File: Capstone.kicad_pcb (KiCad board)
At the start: 2 copper layers, 21 parts, among them U1 XIAO-ESP32-S3-DIP, U2 LM358, U3 LM358, U4 LM358, U5 LM358

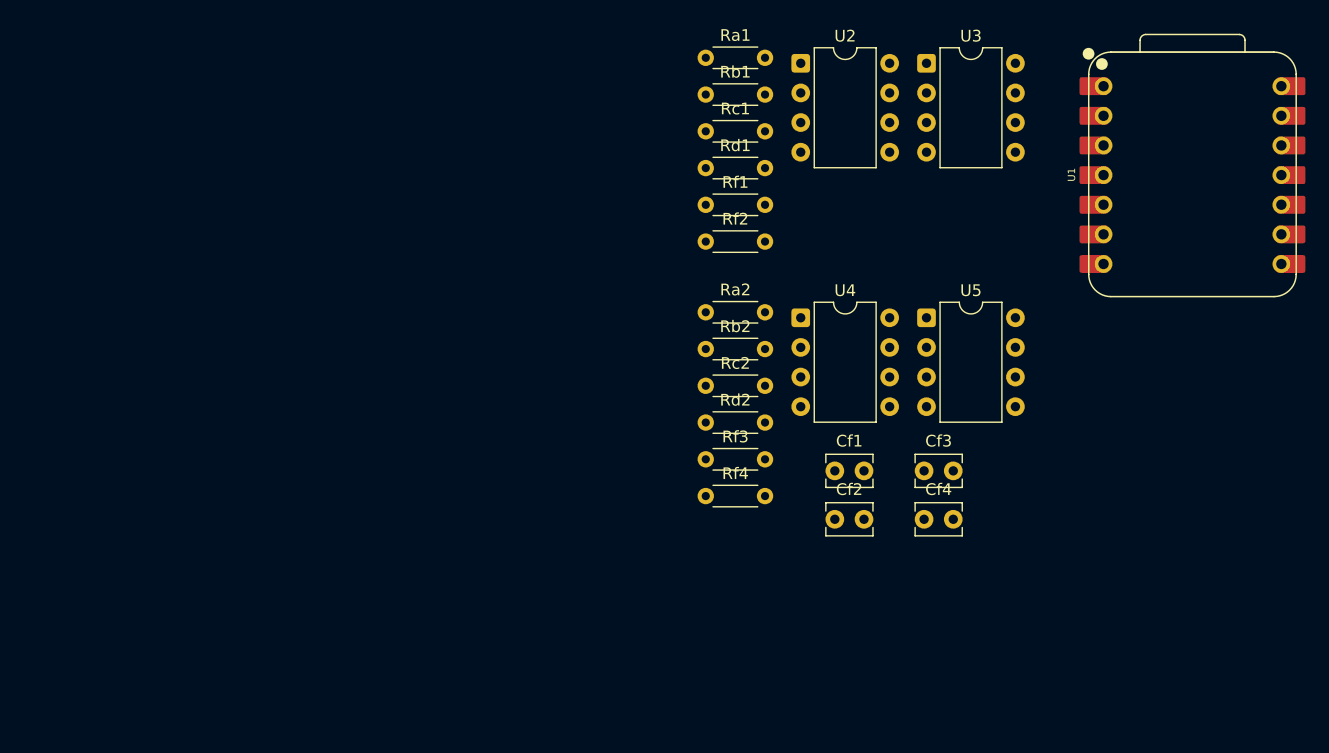
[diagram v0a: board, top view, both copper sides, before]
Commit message: PCB designed rev1.0
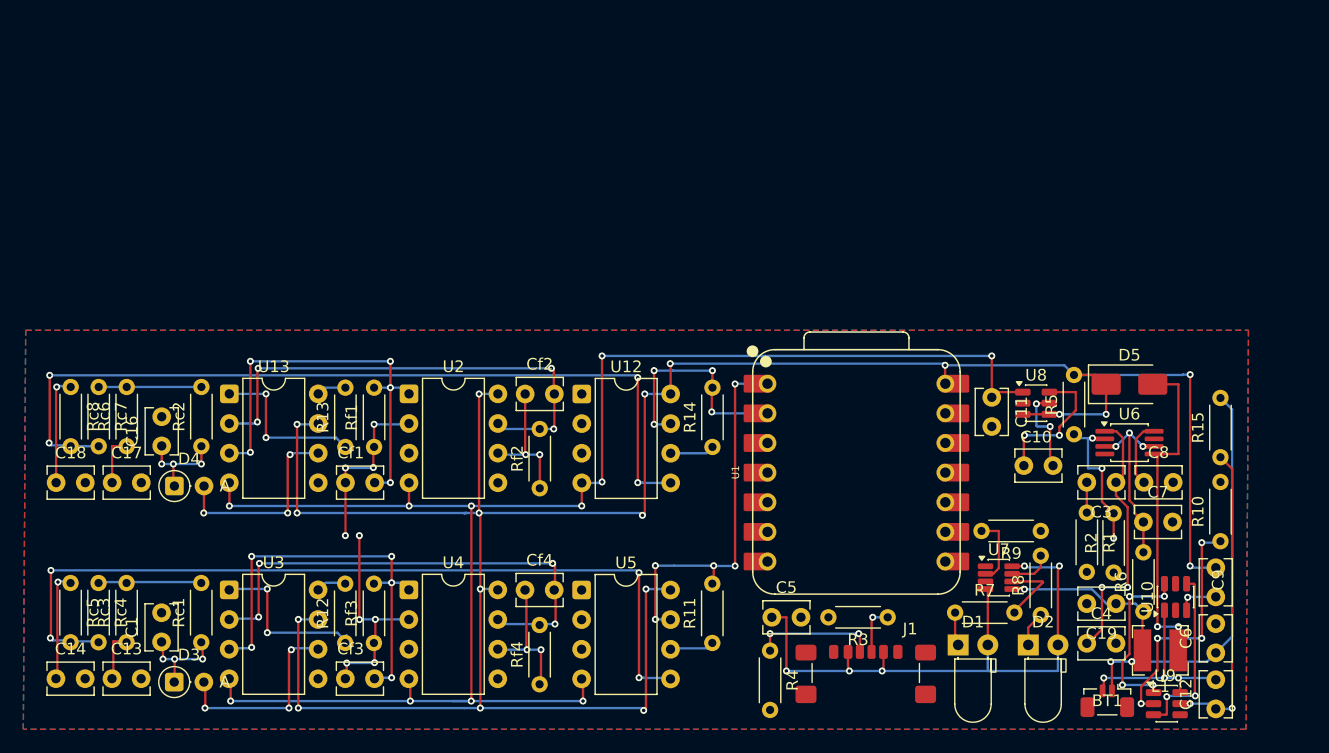
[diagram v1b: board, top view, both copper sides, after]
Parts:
- removed Ra1, Ra2, Rb1, Rb2, Rd1, Rd2: 100k, Resistor_THT:R_Axial_DIN0204_L3.6mm_D1.6mm_P5.08mm_Horizontal
- added BT1: Battery, Connector_JST:JST_SUR_BM02B-SURS-TF_1x02-1MP_P0.80mm_Vertical, F.Cu at (176.7, 125.5)
- added C1: 100p, Capacitor_THT:C_Disc_D3.8mm_W2.6mm_P2.50mm, F.Cu at (95.6, 120.5)
- added C10: 1uF, Capacitor_THT:C_Disc_D3.8mm_W2.6mm_P2.50mm, F.Cu at (172.1, 105.4)
- added C11: 2.2uF, Capacitor_THT:C_Disc_D3.8mm_W2.6mm_P2.50mm, F.Cu at (166.8, 99.5)
- added C12: 100nF, Capacitor_THT:C_Disc_D3.8mm_W2.6mm_P2.50mm, F.Cu at (186.0, 126.2)
- added C13: 100p, Capacitor_THT:C_Disc_D3.8mm_W2.6mm_P2.50mm, F.Cu at (91.4, 123.7)
- added C14: 100p, Capacitor_THT:C_Disc_D3.8mm_W2.6mm_P2.50mm, F.Cu at (86.6, 123.7)
- added C16: 100p, Capacitor_THT:C_Disc_D3.8mm_W2.6mm_P2.50mm, F.Cu at (95.7, 103.7)
- added C17: 100p, Capacitor_THT:C_Disc_D3.8mm_W2.6mm_P2.50mm, F.Cu at (91.4, 106.9)
- added C18: 100p, Capacitor_THT:C_Disc_D3.8mm_W2.6mm_P2.50mm, F.Cu at (86.6, 106.9)
- added C19: 10uF, Capacitor_THT:C_Disc_D3.8mm_W2.6mm_P2.50mm, F.Cu at (177.4, 117.2)
- added C3: 3900pF, Capacitor_THT:C_Disc_D3.8mm_W2.6mm_P2.50mm, F.Cu at (177.4, 106.8)
- added C4: 10pF, Capacitor_THT:C_Disc_D3.8mm_W2.6mm_P2.50mm, F.Cu at (174.9, 120.6)
- added C5: 4.7uF, Capacitor_THT:C_Disc_D3.8mm_W2.6mm_P2.50mm, F.Cu at (147.9, 118.4)
- added C6: 10uF, Capacitor_THT:C_Disc_D3.8mm_W2.6mm_P2.50mm, F.Cu at (186.0, 121.5)
- added C7: 1uF, Capacitor_THT:C_Disc_D3.8mm_W2.6mm_P2.50mm, F.Cu at (179.8, 110.2)
- added C8: 10nF, Capacitor_THT:C_Disc_D3.8mm_W2.6mm_P2.50mm, F.Cu at (179.8, 106.8)
- added C9: 10uF, Capacitor_THT:C_Disc_D3.8mm_W2.6mm_P2.50mm, F.Cu at (186.0, 114.2)
- added D1: LED, LED_THT:LED_D3.0mm_Horizontal_O1.27mm_Z6.0mm, F.Cu at (163.9, 120.8)
- added D2: LED, LED_THT:LED_D3.0mm_Horizontal_O1.27mm_Z6.0mm, F.Cu at (169.9, 120.8)
- added D3: 1N34A, Diode_THT:D_DO-35_SOD27_P2.54mm_Vertical_AnodeUp, F.Cu at (96.7, 124.0)
- added D4: 1N34A, Diode_THT:D_DO-35_SOD27_P2.54mm_Vertical_AnodeUp, F.Cu at (96.7, 107.2)
- added D5: B240A, Diode_SMD:D_SMA, F.Cu at (178.6, 98.4)
- added J1: USB_C_Receptacle_PowerOnly_6P, Connector_USB:USB_C_Receptacle_GCT_USB4135-GF-A_6P_TopMnt_Horizontal, F.Cu at (156.0, 124.4)
- added L1: 3.9uH, Inductor_SMD:L_Bourns-SRN4018, F.Cu at (181.2, 121.2)
- added R1: 4.75k, Resistor_THT:R_Axial_DIN0204_L3.6mm_D1.6mm_P5.08mm_Horizontal, F.Cu at (174.9, 109.4)
- added R10: 1k, Resistor_THT:R_Axial_DIN0204_L3.6mm_D1.6mm_P5.08mm_Horizontal, F.Cu at (186.4, 111.9)
- added R11: 1k, Resistor_THT:R_Axial_DIN0204_L3.6mm_D1.6mm_P5.08mm_Horizontal, F.Cu at (142.8, 120.6)
- added R12: 500, Resistor_THT:R_Axial_DIN0204_L3.6mm_D1.6mm_P5.08mm_Horizontal, F.Cu at (111.4, 120.6)
- added R13: 500, Resistor_THT:R_Axial_DIN0204_L3.6mm_D1.6mm_P5.08mm_Horizontal, F.Cu at (111.4, 103.8)
- added R14: 1k, Resistor_THT:R_Axial_DIN0204_L3.6mm_D1.6mm_P5.08mm_Horizontal, F.Cu at (142.9, 103.8)
- added R15: 100R, Resistor_THT:R_Axial_DIN0204_L3.6mm_D1.6mm_P5.08mm_Horizontal, F.Cu at (186.4, 104.7)
- added R2: 33.2K, Resistor_THT:R_Axial_DIN0204_L3.6mm_D1.6mm_P5.08mm_Horizontal, F.Cu at (177.2, 114.6)
- added R3: 5.11k, Resistor_THT:R_Axial_DIN0204_L3.6mm_D1.6mm_P5.08mm_Horizontal, F.Cu at (157.9, 118.4)
- added R4: 5.11k, Resistor_THT:R_Axial_DIN0204_L3.6mm_D1.6mm_P5.08mm_Horizontal, F.Cu at (147.8, 121.3)
- added R5: 102k, Resistor_THT:R_Axial_DIN0204_L3.6mm_D1.6mm_P5.08mm_Horizontal, F.Cu at (173.8, 102.7)
- added R6: 1, Resistor_THT:R_Axial_DIN0204_L3.6mm_D1.6mm_P5.08mm_Horizontal, F.Cu at (179.8, 117.9)
- added R7: 5.11k, Resistor_THT:R_Axial_DIN0204_L3.6mm_D1.6mm_P5.08mm_Horizontal, F.Cu at (163.7, 118.0)
- added R8: 5.11k, Resistor_THT:R_Axial_DIN0204_L3.6mm_D1.6mm_P5.08mm_Horizontal, F.Cu at (171.0, 118.2)
- added R9: 5.11k, Resistor_THT:R_Axial_DIN0204_L3.6mm_D1.6mm_P5.08mm_Horizontal, F.Cu at (171.0, 111.0)
- added Rc3: 1k, Resistor_THT:R_Axial_DIN0204_L3.6mm_D1.6mm_P5.08mm_Horizontal, F.Cu at (92.6, 120.5)
- added Rc4: 100k, Resistor_THT:R_Axial_DIN0204_L3.6mm_D1.6mm_P5.08mm_Horizontal, F.Cu at (90.2, 115.5)
- added Rc5: 1k, Resistor_THT:R_Axial_DIN0204_L3.6mm_D1.6mm_P5.08mm_Horizontal, F.Cu at (87.8, 115.5)
- added Rc6: 1k, Resistor_THT:R_Axial_DIN0204_L3.6mm_D1.6mm_P5.08mm_Horizontal, F.Cu at (92.7, 103.7)
- added Rc7: 100k, Resistor_THT:R_Axial_DIN0204_L3.6mm_D1.6mm_P5.08mm_Horizontal, F.Cu at (90.3, 98.7)
- added Rc8: 1k, Resistor_THT:R_Axial_DIN0204_L3.6mm_D1.6mm_P5.08mm_Horizontal, F.Cu at (87.9, 98.7)
- added U10: ~, Package_TO_SOT_SMD:SOT-23-6, F.Cu at (182.6, 116.7)
- added U12: LM358, Package_DIP:DIP-8_W7.62mm, F.Cu at (131.7, 99.3)
- added U13: INA128, Package_DIP:DIP-8_W7.62mm, F.Cu at (101.5, 99.2)
- added U6: ADP1613ARMZ-R7, Package_SO:MSOP-8_3x3mm_P0.65mm, F.Cu at (178.6, 103.4)
- added U7: ~, Package_TO_SOT_SMD:SOT-23-8, F.Cu at (167.4, 115.0)
- added U8: LM2776, Package_TO_SOT_SMD:SOT-23-6, F.Cu at (170.6, 100.0)
- added U9: ~, Package_TO_SOT_SMD:SOT-23-6, F.Cu at (181.8, 125.8)
- Cf1, Cf3: value 10p -> 2p
- U3: value LM358 -> INA128
- moved U3 74.9 mm to (101.4, 116.0)
- moved Rc1 61.5 mm to (99.0, 120.5), turned to 90 degrees
- moved Cf3 52.7 mm to (111.4, 123.7)
- moved U2 43.9 mm to (116.9, 99.2)
- moved Rc2 43.5 mm to (99.1, 103.7), turned to 90 degrees
- moved Cf1 42.0 mm to (111.4, 106.9)
- moved U4 40.9 mm to (116.8, 116.0)
- moved U1 38.5 mm to (155.2, 106.0)
- moved U5 37.7 mm to (131.6, 116.1)
- moved Rf1 35.2 mm to (113.9, 103.8), turned to 90 degrees
- moved Cf4 34.7 mm to (126.8, 116.1)
- moved Rf3 32.5 mm to (113.8, 120.6), turned to 90 degrees
- moved Cf2 28.6 mm to (126.8, 99.3)
- moved Rf2 25.5 mm to (128.1, 107.3), turned to 90 degrees
- moved Rf4 21.5 mm to (128.0, 124.1), turned to 90 degrees
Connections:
- net /SensorReader/V- renamed -5V_OUT
- Rc1 pad 1: Net-(U3A--) -> Net-(D3-K)
- Rc1 pad 2: /SensorReader1/Vout -> Net-(Rc1-Pad2)
- Rc2 pad 1: Net-(U5A--) -> Net-(D4-K)
- Rc2 pad 2: /SensorReader/Vout -> Net-(Rc2-Pad2)
- U1 pad 13: /SensorReader/Vref -> GND
- U1 pad 14: /SensorReader/V+ -> 5V OUT
- U2 pad 3: /SensorReader/Vref -> GND
- U2 pad 5: /SensorReader/Vref -> GND
- U2 pad 8: /SensorReader/V+ -> 5V OUT
- U3 pad 1: /SensorReader1/Vout -> Net-(R12-Pad1)
- U3 pad 2: Net-(U3A--) -> /SensorReader/V2
- U3 pad 3: Net-(U3A-+) -> /SensorReader/V1
- U3 pad 5: unconnected-(U3B-+-Pad5) -> GND
- U3 pad 6: unconnected-(U3B---Pad6) -> Net-(D3-A)
- U3 pad 7: unconnected-(U3-Pad7) -> 5V OUT
- U3 pad 8: /SensorReader/V+ -> Net-(R12-Pad2)
- U4 pad 3: /SensorReader/Vref -> GND
- U4 pad 5: /SensorReader/Vref -> GND
- U4 pad 8: /SensorReader/V+ -> 5V OUT
- U5 pad 1: /SensorReader/Vout -> (no net)
- U5 pad 2: Net-(U5A--) -> (no net)
- U5 pad 3: Net-(U5A-+) -> (no net)
- U5 pad 5: unconnected-(U5B-+-Pad5) -> Net-(U5B-+)
- U5 pad 6: unconnected-(U5B---Pad6) -> Net-(U5B--)
- U5 pad 7: unconnected-(U5-Pad7) -> /SensorReader/Vout
- U5 pad 8: /SensorReader/V+ -> 5V OUT
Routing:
- net 5V OUT: track 0.00 -> 214.8 mm, vias 0 -> 18
- net -5V_OUT: track 0.00 -> 143.0 mm, vias 0 -> 11
- net Net-(U5B-+): track 0.00 -> 72.5 mm, vias 0 -> 4
- net Net-(U12B-+): track 0.00 -> 72.5 mm, vias 0 -> 4
- net Net-(D1-A): track 0.00 -> 53.0 mm, vias 0 -> 5
- net B+: track 0.00 -> 51.6 mm, vias 0 -> 3
- net /SensorReader1/V2: track 0.00 -> 42.6 mm, vias 0 -> 4
- net /SensorReader/V2: track 0.00 -> 42.6 mm, vias 0 -> 4
- net /SensorReader1/V1: track 0.00 -> 36.8 mm, vias 0 -> 5
- net /SensorReader/V1: track 0.00 -> 36.8 mm, vias 0 -> 5
- net /SensorReader/Vout: track 0.00 -> 33.0 mm, vias 0 -> 5
- net Net-(D5-A): track 0.00 -> 29.0 mm, vias 0 -> 2
- net Net-(U9-VCC): track 0.00 -> 27.2 mm, vias 0 -> 2
- net Net-(U6-COMP): track 0.00 -> 22.8 mm, vias 0 -> 2
- net Net-(U9-CS): track 0.00 -> 20.9 mm, vias 0 -> 4
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- added copper zone on B.Cu, net GND
- added copper zone on F.Cu, net GND
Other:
- board text added: "${REFERENCE}"
